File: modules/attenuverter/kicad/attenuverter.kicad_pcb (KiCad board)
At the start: 2 copper layers, 28 x 108 mm, 23 parts, among them J1 IN 1, J2 OUT 1, J3 IN 2, J4 OUT 2, J5 POWER, U1 TL072

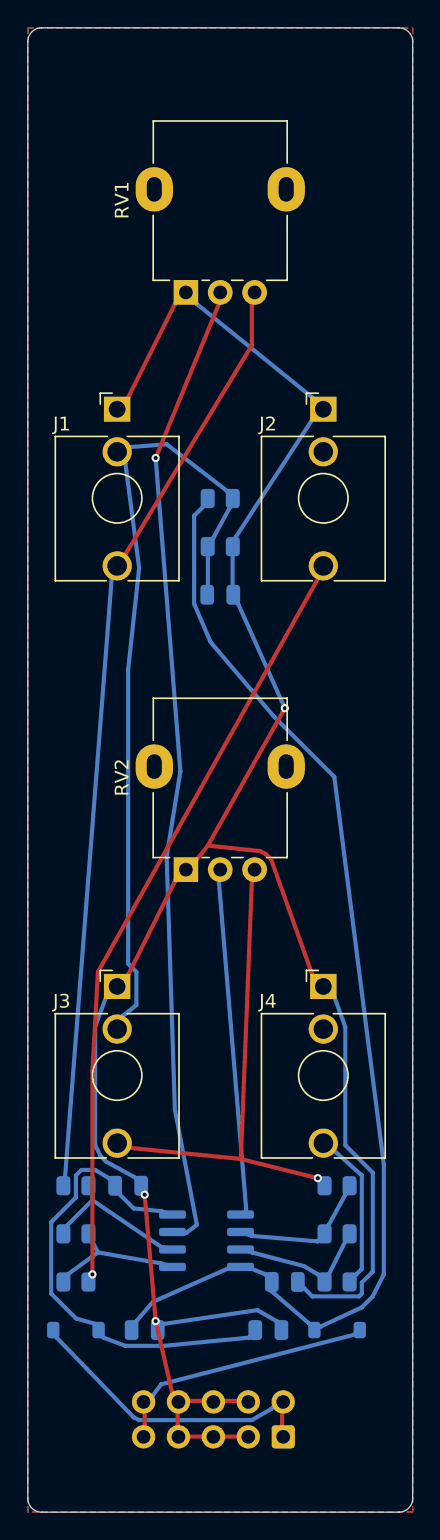
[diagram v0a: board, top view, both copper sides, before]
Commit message: M1-M3: reject invalid designs, forbid vias in pads, fail closed on export
Three of the roadmap's review findings become code and tests. Every design
is now validated before emission, the router's result is checked on the
final geometry rather than trusted, and nothing can be exported that a
clean check did not produce.

Validation (toolkit/src/Validate.hs, wired into pcbgen before emission):
unique references and net names, every (ref, pin) must exist on the library
symbol, every symbol pin must be on exactly one net or listed in the new
partNoConnect, assembly class and LCSC field must agree, dimensions and
routing settings must be positive. On any diagnostic pcbgen prints them and
exits 1 without writing a file. The four wiring faults ERC used to accept
(U1.8 removed, mistyped as U1.88, on both rails, D2.1 dropped) are rejected
with diagnostics that name the pin.

Routing (toolkit/src/Route/Check.hs, Router.hs): a via may no longer be
placed in or against any pad, its own net included, which is what put 0.3 mm
drills in four SMD solder lands. Pre-routed copper is treated as one terminal
per island, so a hand-drawn trace can no longer make a net look finished
while a pad hangs unconnected, and it now blocks by its own width. Per-net
connectivity and via/pad clearance are recomputed on the emitted geometry;
any failure, contested cell or disconnect aborts generation.

Pours: Zone gains an explicit PadConnect. The attenuverter routes GND as
copper, so its pours no longer bond to pads at all, which also removes the
starved-thermal violation the stricter routing exposed. The mult's sleeves
are held by its pours alone and keep thermal relief; validation rejects an
unbonded pour on a net nothing routes.

Scripts: check.sh writes build/check.ok (tool versions, git provenance,
sha256 of every source and of the zone-filled board) only when ERC and DRC
are both clean, and removes stale copies first. fab.sh refuses unless every
hash still matches, builds into a temporary dire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
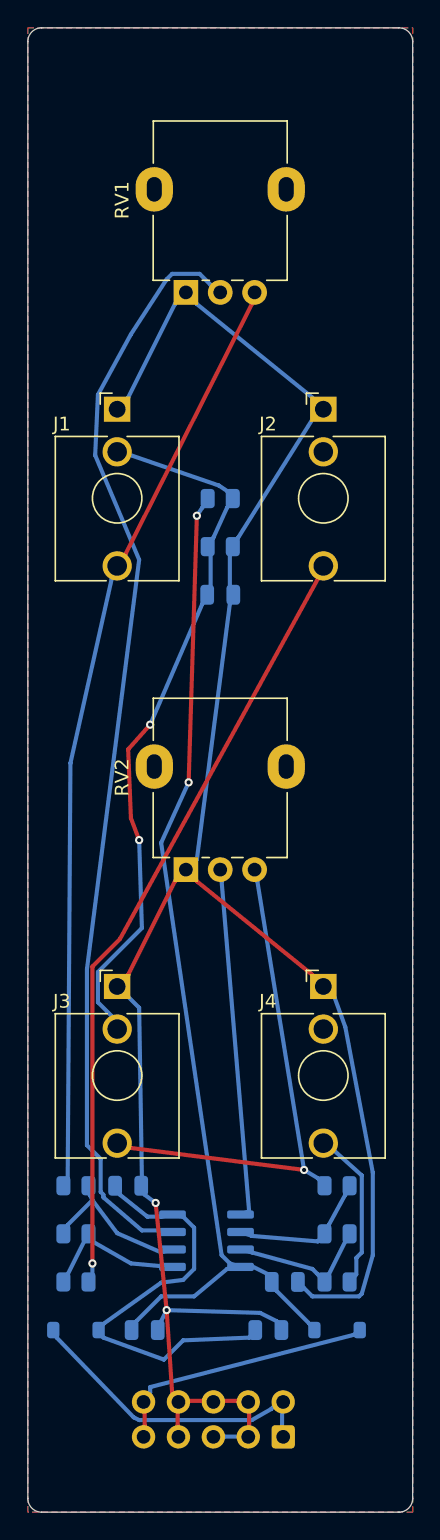
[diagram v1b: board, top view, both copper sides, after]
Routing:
- net +12V: track 84.6 -> 75.0 mm, vias 0 -> 2
- net /WIPER1: track 71.1 -> 80.1 mm, vias 1 -> 0
- net /OFFSET: track 60.5 -> 51.8 mm, vias 0 -> 2
- net GND: track 171.5 -> 167.0 mm, vias 3 -> 2
- net -12V: track 34.4 -> 31.4 mm
- net /IN2: track 36.7 -> 37.8 mm
